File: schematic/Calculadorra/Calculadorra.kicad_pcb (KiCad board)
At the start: 2 copper layers, 20 parts, among them SW1 SW_Push, SW10 SW_Push, SW11 SW_Push, SW12 SW_Push, SW13 SW_Push, SW14 SW_Push, SW15 SW_Push, SW16 SW_Push, SW2 SW_Push, SW3 SW_Push, SW4 SW_Push, SW5 SW_Push, SW6 SW_Push, SW7 SW_Push, SW8 SW_Push, SW9 SW_Push, U1 ATmega328-P, U2 LCD-016N002L

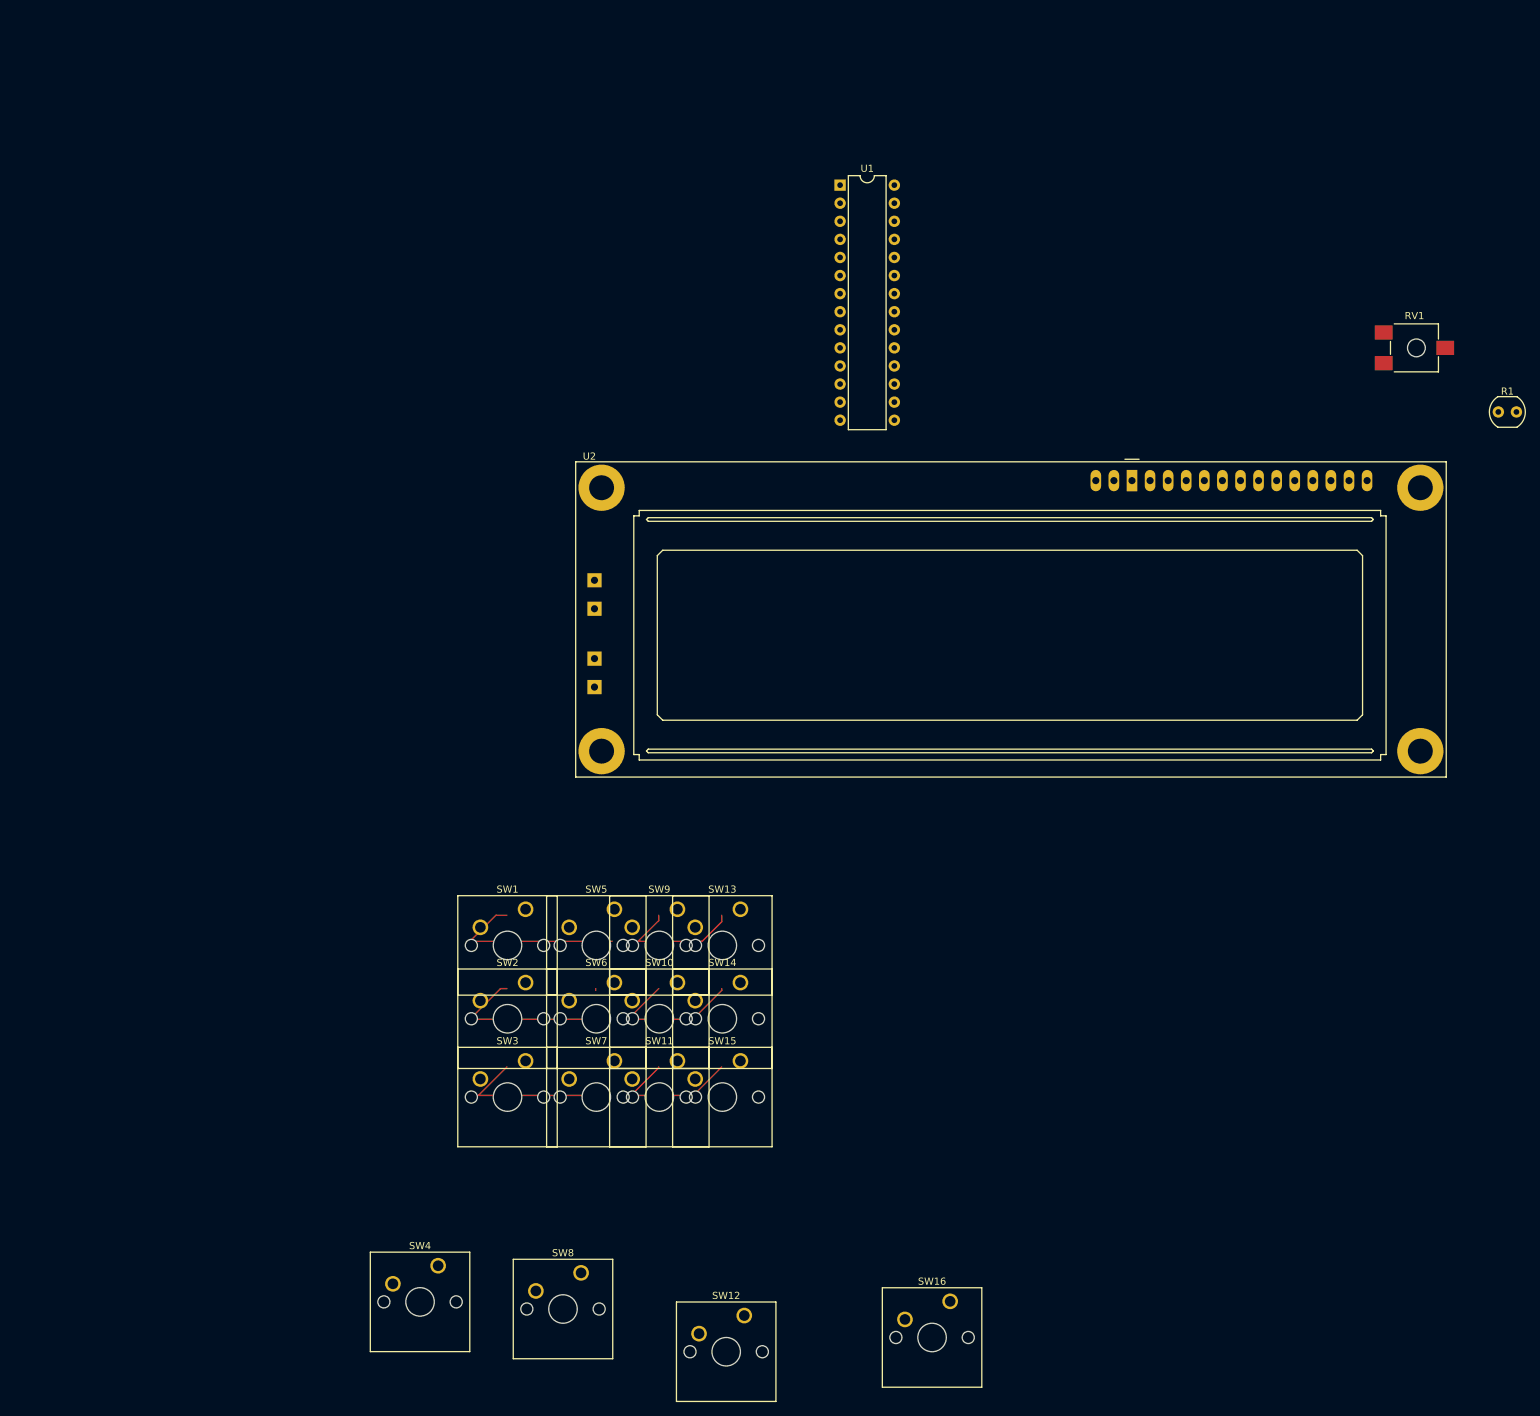
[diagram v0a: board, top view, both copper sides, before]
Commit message: No idea what changed
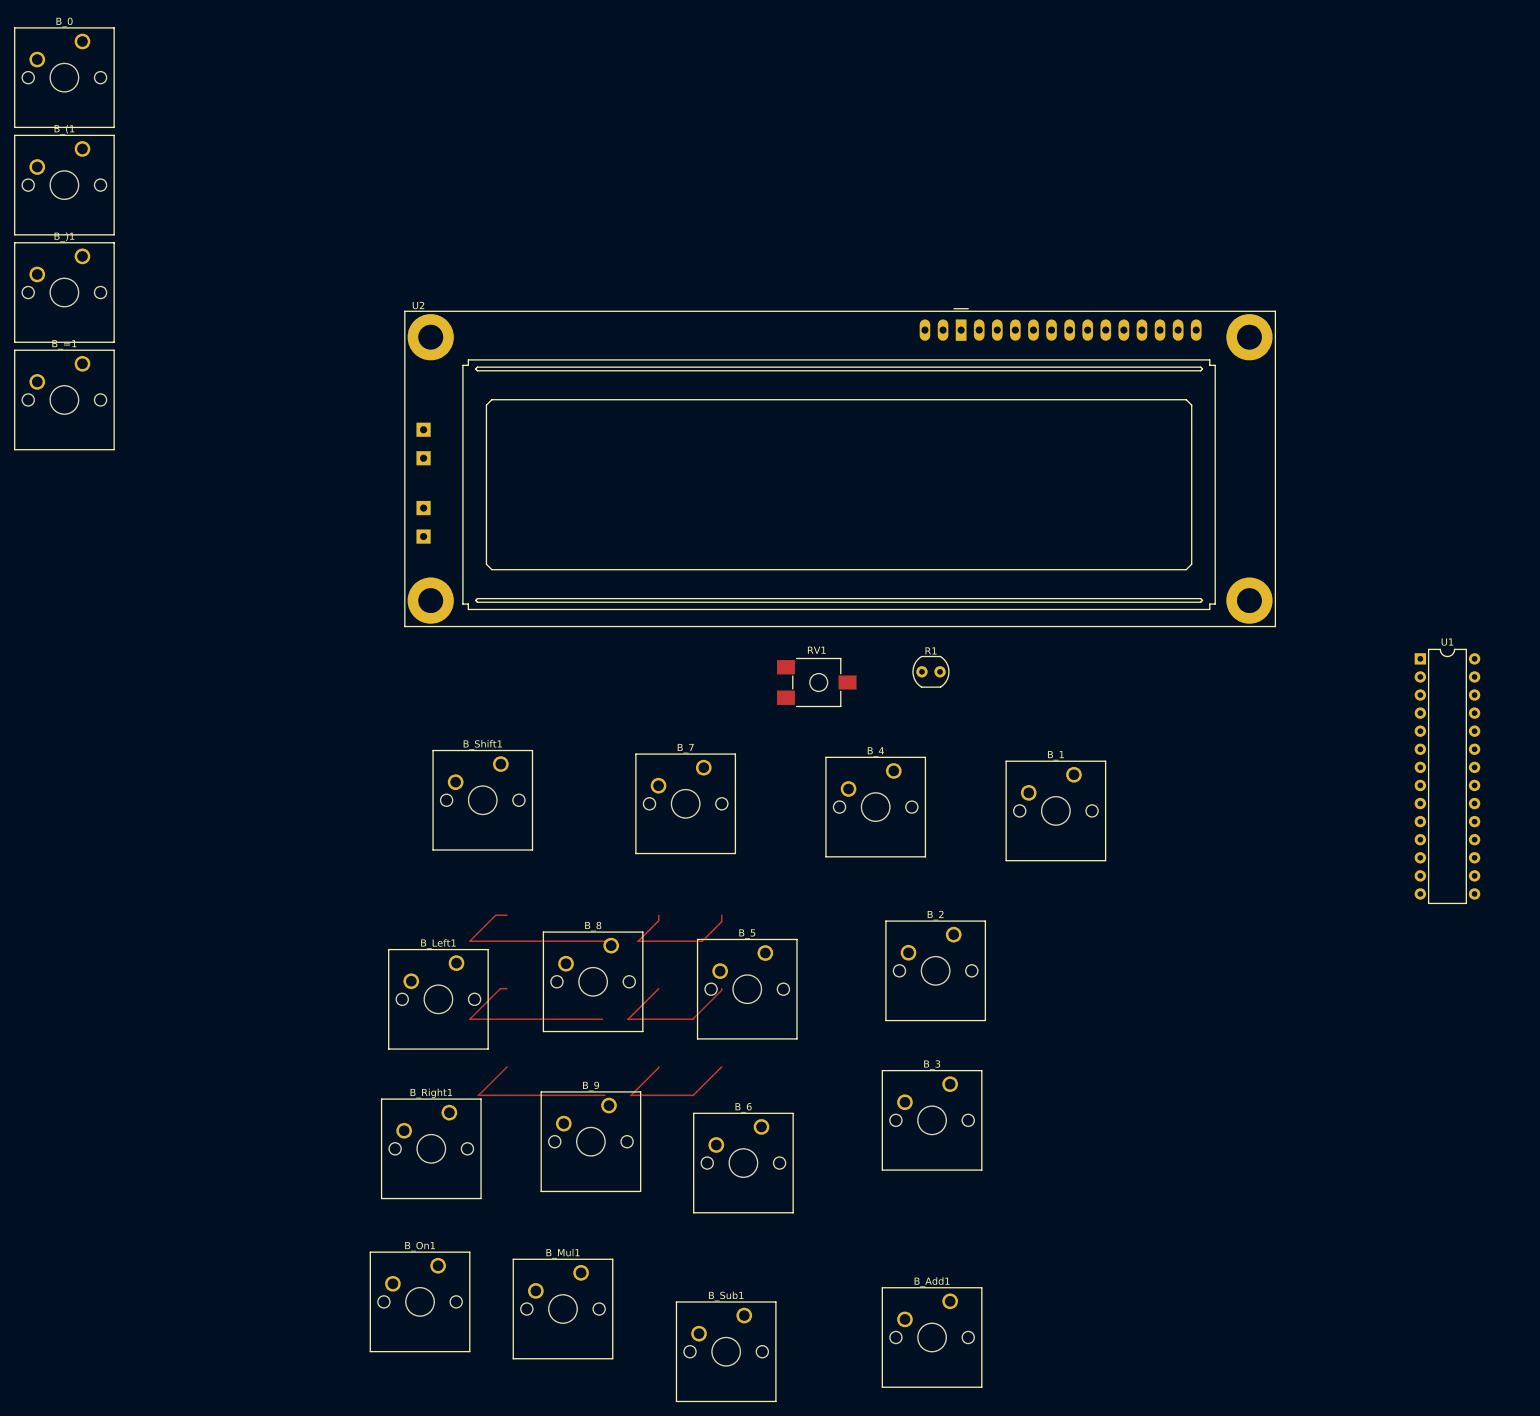
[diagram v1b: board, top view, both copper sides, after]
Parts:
- added B_(1: SW_Push, Button_Switch_Keyboard:SW_Cherry_MX_1.00u_PCB, F.Cu at (9.59, 17.1)
- added B_)1: SW_Push, Button_Switch_Keyboard:SW_Cherry_MX_1.00u_PCB, F.Cu at (9.59, 32.1)
- added B_0: SW_Push, Button_Switch_Keyboard:SW_Cherry_MX_1.00u_PCB, F.Cu at (9.59, 1.97)
- added B_=1: SW_Push, Button_Switch_Keyboard:SW_Cherry_MX_1.00u_PCB, F.Cu at (9.59, 47.2)
- moved U1 105.2 mm to (197.5, 88.7)
- moved RV1 96.2 mm to (112.7, 92.0)
- moved R1 88.8 mm to (127.5, 90.5)
- moved B_1 50.5 mm to (148.8, 105.0)
- moved B_4 36.1 mm to (123.5, 104.4)
- moved U2 32.0 mm to (133.0, 42.5)
- moved B_2 30.7 mm to (132.0, 127.4)
- moved B_3 29.6 mm to (131.5, 148.4)
- moved B_7 23.5 mm to (96.8, 104.0)
- moved B_Shift1 20.7 mm to (68.3, 103.5)
- moved B_6 15.0 mm to (105.0, 154.4)
- moved B_5 13.0 mm to (105.5, 130.0)
- moved B_Right1 12.9 mm to (61.1, 152.4)
- moved B_Left1 10.1 mm to (62.1, 131.4)
- moved B_9 6.32 mm to (83.5, 151.4)
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- renumbered SW13 to B_1, SW14 to B_2, SW15 to B_3, SW9 to B_4, SW10 to B_5, SW11 to B_6, SW5 to B_7, SW6 to B_8, SW7 to B_9, SW16 to B_Add1, SW2 to B_Left1, SW8 to B_Mul1, SW4 to B_On1, SW3 to B_Right1, SW1 to B_Shift1, SW12 to B_Sub1
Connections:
- B_1 pad 1: Net-(U1-PD3) -> Net-(U1-PD2)
- B_2 pad 1: Net-(U1-PD3) -> Net-(U1-PD2)
- B_3 pad 1: Net-(U1-PD3) -> Net-(U1-PD2)
- B_4 pad 1: Net-(U1-PD2) -> Net-(U1-PD1)
- B_5 pad 1: Net-(U1-PD2) -> Net-(U1-PD1)
- B_6 pad 1: Net-(U1-PD2) -> Net-(U1-PD1)
- B_7 pad 1: Net-(U1-PD1) -> Net-(U1-PD0)
- B_8 pad 1: Net-(U1-PD1) -> Net-(U1-PD0)
- B_9 pad 1: Net-(U1-PD1) -> Net-(U1-PD0)
- B_Add1 pad 1: Net-(U1-PD3) -> Net-(U1-PD2)
- B_Left1 pad 1: Net-(U1-PD0) -> Net-(U1-PC5)
- B_Mul1 pad 1: Net-(U1-PD1) -> Net-(U1-PD0)
- B_On1 pad 1: Net-(U1-PD0) -> Net-(U1-PC5)
- B_Right1 pad 1: Net-(U1-PD0) -> Net-(U1-PC5)
- B_Shift1 pad 1: Net-(U1-PD0) -> Net-(U1-PC5)
- B_Sub1 pad 1: Net-(U1-PD2) -> Net-(U1-PD1)
- U1 pad 28: unconnected-(U1-PC5-Pad28) -> Net-(U1-PC5)
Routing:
- net Net-(U1-PD4): track 45.4 -> 18.6 mm
- net Net-(U1-PD0): track 0.00 -> 26.7 mm

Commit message: Disseny de la PCB i model 3D fet durant la Hacknight
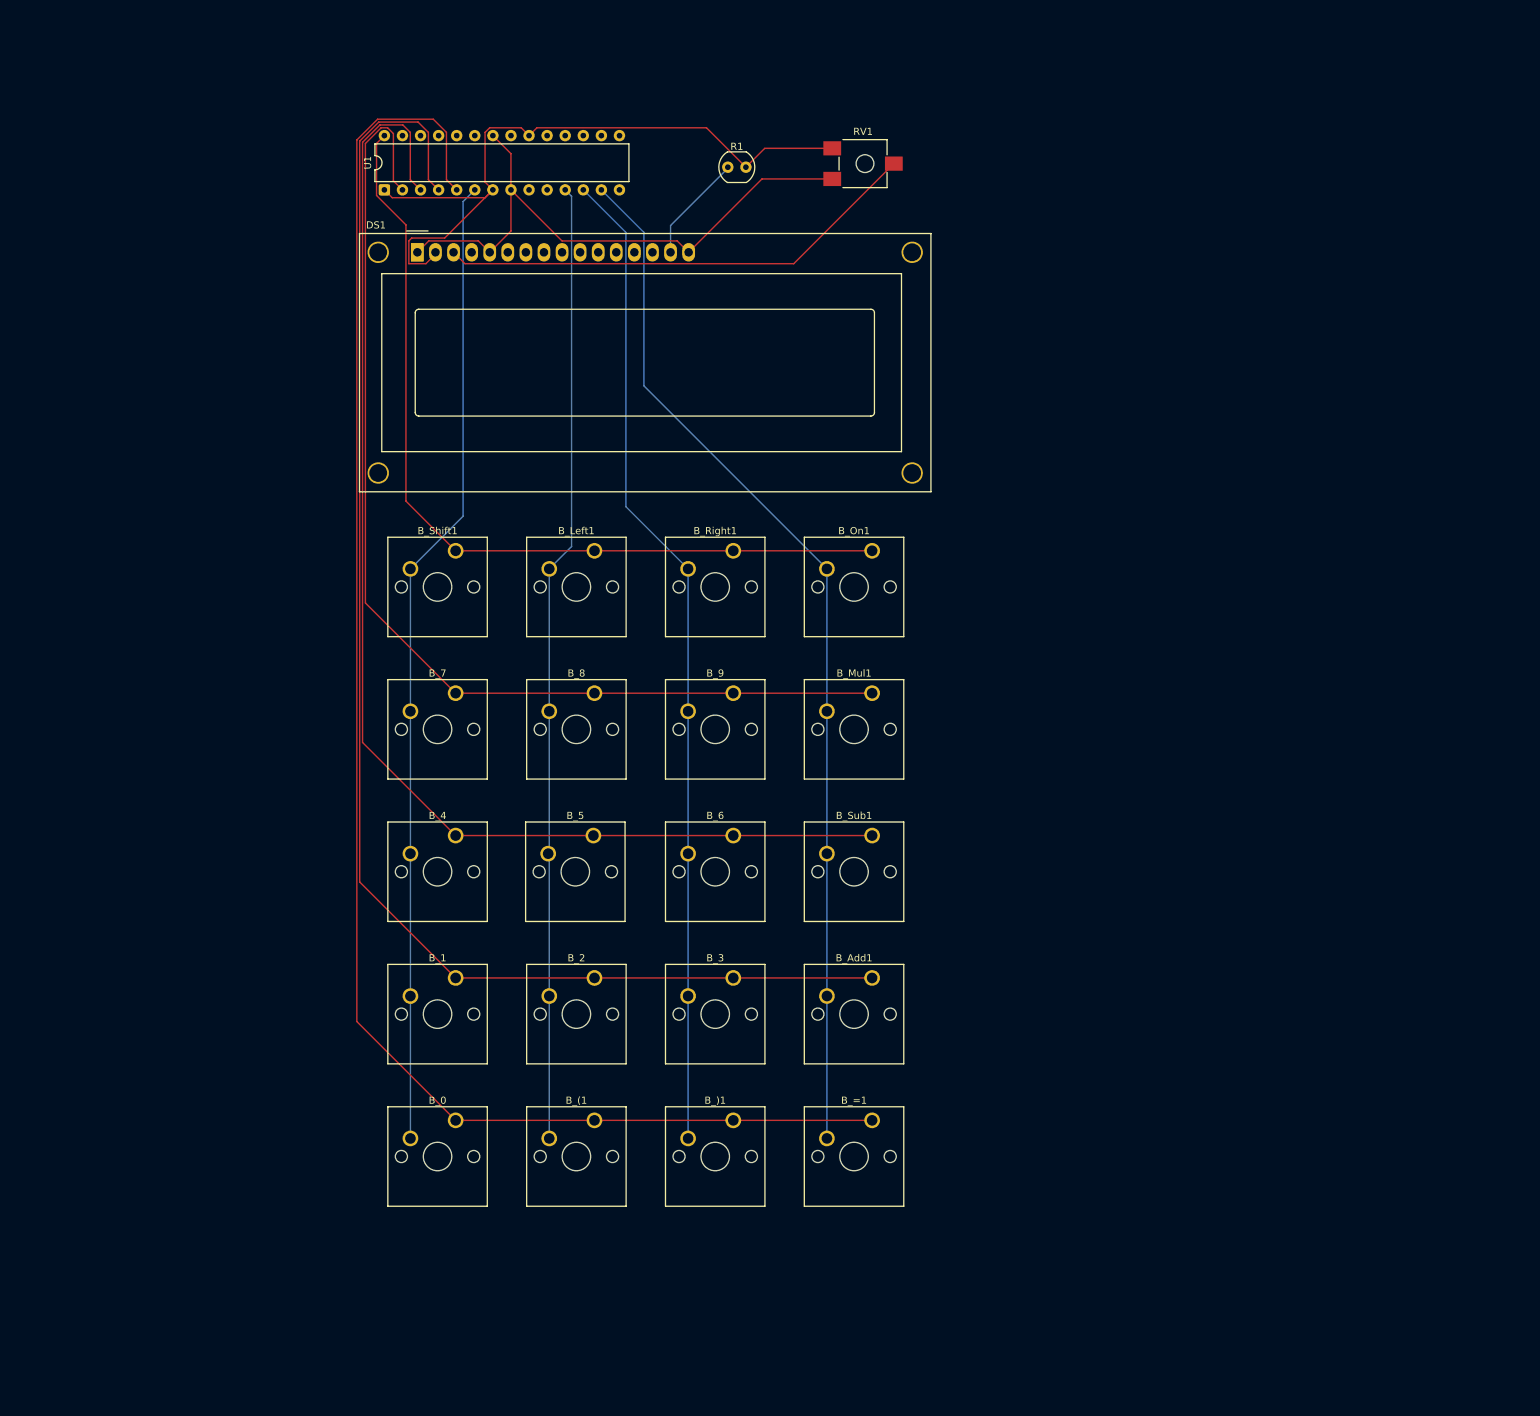
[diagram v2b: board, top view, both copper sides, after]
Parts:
- removed U2: LCD-016N002L, Display:LCD-016N002L
- added DS1: WC1602A, Display:WC1602A, F.Cu at (56.6, 31.6)
- moved B_0 160.3 mm to (62.0, 153.5)
- moved U1 159.7 mm to (52.0, 22.8), turned to 90 degrees
- moved B_(1 154.2 mm to (81.5, 153.5)
- moved B_=1 153.6 mm to (120.5, 153.5)
- moved B_)1 151.9 mm to (101.0, 153.5)
- moved B_On1 117.5 mm to (120.5, 73.5)
- moved B_1 91.4 mm to (62.0, 133.5)
- moved B_Mul1 91.1 mm to (120.5, 93.5)
- moved B_Right1 88.4 mm to (101.0, 73.5)
- moved R1 75.9 mm to (100.2, 19.6)
- moved RV1 73.2 mm to (119.2, 19.1)
- moved B_Sub1 69.8 mm to (120.5, 113.5)
- moved B_4 62.2 mm to (62.0, 113.5)
- moved B_Left1 61.1 mm to (81.5, 73.5)
- moved B_9 60.5 mm to (101.0, 93.5)
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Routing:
- net Net-(U1-PD3): track 0.00 -> 225.2 mm
- net Net-(U1-PD2): track 0.00 -> 201.7 mm
- net Net-(U1-PD1): track 0.00 -> 178.1 mm
- net Net-(U1-PD7): track 0.00 -> 146.4 mm
- net Net-(U1-PD0): track 26.7 -> 154.6 mm
- net Net-(U1-PC5): track 0.00 -> 121.9 mm
- net Net-(U1-PD4): track 18.6 -> 137.0 mm
- net VCC: track 0.00 -> 100.6 mm
- net Net-(U1-PD6): track 43.5 -> 139.3 mm
- net Net-(U1-PD5): track 47.0 -> 135.0 mm
- net GND: track 0.00 -> 83.2 mm
- net Net-(DS1-VO): track 0.00 -> 68.3 mm
- net Net-(DS1-D7): track 0.00 -> 32.3 mm
- net Net-(DS1-RS): track 0.00 -> 28.1 mm
- net Net-(DS1-D6): track 0.00 -> 28.0 mm
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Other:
- copper layers 2 -> 4
